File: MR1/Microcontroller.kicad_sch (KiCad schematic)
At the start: 28 parts, among them J22 B4B_PH, J23 Jumper_1, J36 Conn_ARM_JTAG_SWD_10, SW1 SW_Push, SW2 SW_Push, U8 ESP32-S3-MINI-1U, Y2 32.768 kHz

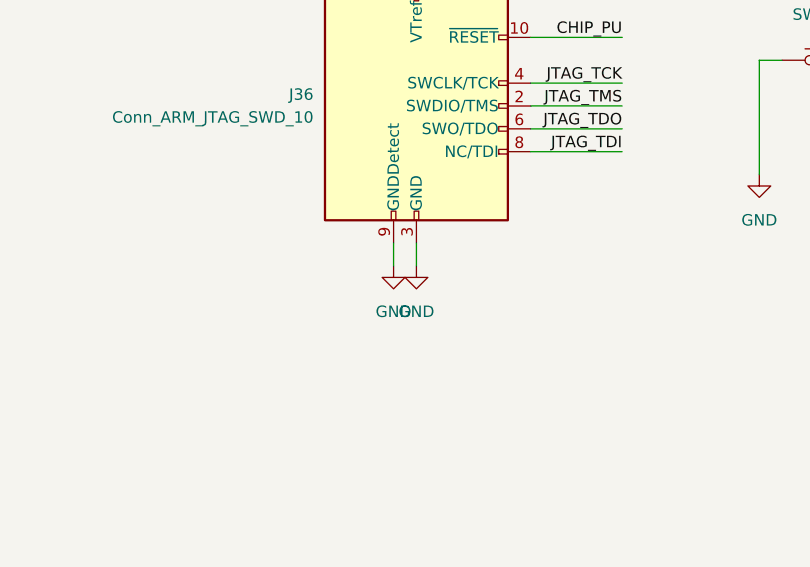
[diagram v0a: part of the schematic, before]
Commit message: Signed-off-by: lokimetasmith <lokimail@gmail.com>
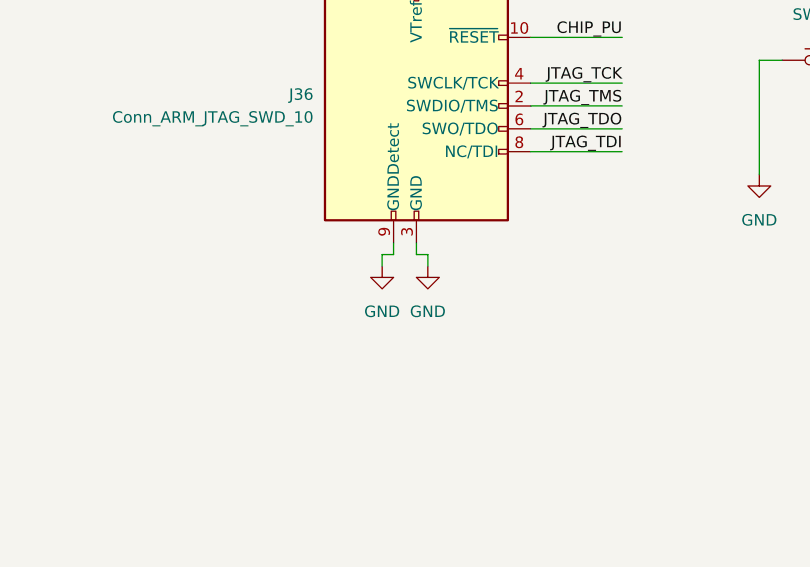
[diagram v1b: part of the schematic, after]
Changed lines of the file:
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@@
 	(wire
 		(pts
+			(xy 170.18 148.59) (xy 168.91 148.59)
+		)
+		(stroke
+			(width 0)
+			(type default)
+		)
+	)
+	(wire
+		(pts
 			(xy 49.53 104.14) (xy 57.15 104.14)
 		)
@@
 	(wire
 		(pts
-			(xy 168.91 147.32) (xy 168.91 149.86)
+			(xy 170.18 148.59) (xy 170.18 149.86)
 		)
 		(stroke
@@
 	(wire
 		(pts
+			(xy 165.1 148.59) (xy 166.37 148.59)
+		)
+		(stroke
+			(width 0)
+			(type default)
+		)
+	)
+	(wire
+		(pts
+			(xy 166.37 148.59) (xy 166.37 147.32)
+		)
+		(stroke
+			(width 0)
+			(type default)
+		)
+	)
+	(wire
+		(pts
 			(xy 154.94 53.34) (xy 180.34 53.34)
 		)
@@
 	(wire
 		(pts
+			(xy 168.91 148.59) (xy 168.91 147.32)
+		)
+		(stroke
+			(width 0)
+			(type default)
+		)
+	)
+	(wire
+		(pts
 			(xy 210.82 66.04) (xy 238.76 66.04)
 		)
@@
 	(wire
 		(pts
-			(xy 166.37 147.32) (xy 166.37 149.86)
+			(xy 165.1 148.59) (xy 165.1 149.86)
 		)
 		(stroke
@@
 	(symbol
 		(lib_id "power:GND")
-		(at 168.91 149.86 0)
+		(at 170.18 149.86 0)
 		(unit 1)
 		(body_style 1)
@@
 		(fields_autoplaced yes)
 		(property "Reference" "#PWR0139"
-			(at 168.91 156.21 0)
+			(at 170.18 156.21 0)
 			(hide yes)
 			(show_name no)
@@
 		)
 		(property "Value" "GND"
-			(at 168.91 154.94 0)
+			(at 170.18 154.94 0)
 			(show_name no)
 			(do_not_autoplace no)
@@
 		)
 		(property "Footprint" ""
-			(at 168.91 149.86 0)
+			(at 170.18 149.86 0)
 			(hide yes)
 			(show_name no)
@@
 		)
 		(property "Datasheet" ""
-			(at 168.91 149.86 0)
+			(at 170.18 149.86 0)
 			(hide yes)
 			(show_name no)
@@
 		)
 		(property "Description" "Power symbol creates a global label with name \"GND\" , ground"
-			(at 168.91 149.86 0)
+			(at 170.18 149.86 0)
 			(hide yes)
 			(show_name no)
@@
 	(symbol
 		(lib_id "power:GND")
-		(at 166.37 149.86 0)
+		(at 165.1 149.86 0)
 		(unit 1)
 		(body_style 1)
@@
 		(fields_autoplaced yes)
 		(property "Reference" "#PWR0138"
-			(at 166.37 156.21 0)
+			(at 165.1 156.21 0)
 			(hide yes)
 			(show_name no)
@@
 		)
 		(property "Value" "GND"
-			(at 166.37 154.94 0)
+			(at 165.1 154.94 0)
 			(show_name no)
 			(do_not_autoplace no)
@@
 		)
 		(property "Footprint" ""
-			(at 166.37 149.86 0)
+			(at 165.1 149.86 0)
 			(hide yes)
 			(show_name no)
@@
 		)
 		(property "Datasheet" ""
-			(at 166.37 149.86 0)
+			(at 165.1 149.86 0)
 			(hide yes)
 			(show_name no)
@@
 		)
 		(property "Description" "Power symbol creates a global label with name \"GND\" , ground"
-			(at 166.37 149.86 0)
+			(at 165.1 149.86 0)
 			(hide yes)
 			(show_name no)
